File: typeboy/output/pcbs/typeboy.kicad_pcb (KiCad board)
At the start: 2 copper layers, 141.2 x 105.6 mm, 66 parts, among them J2 CartBus

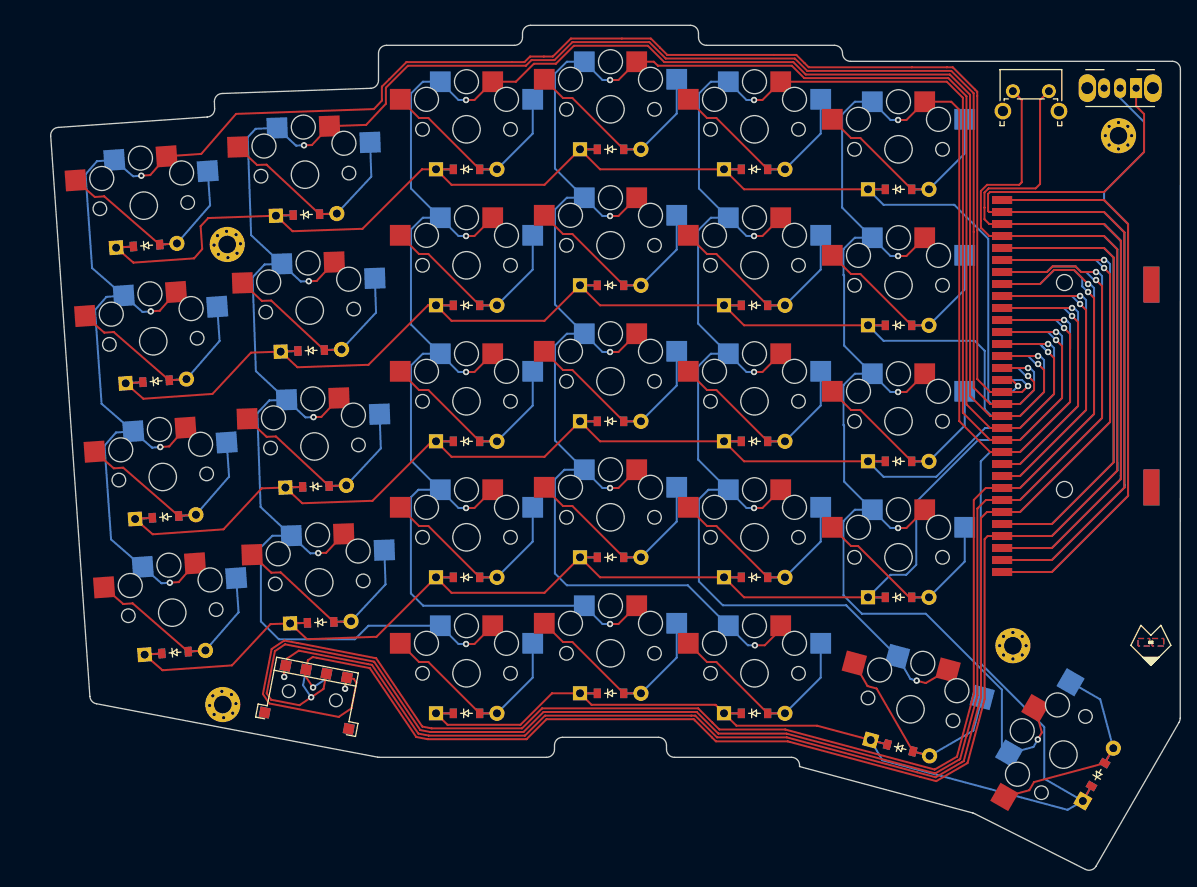
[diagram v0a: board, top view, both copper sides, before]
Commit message: Updated Documentation.
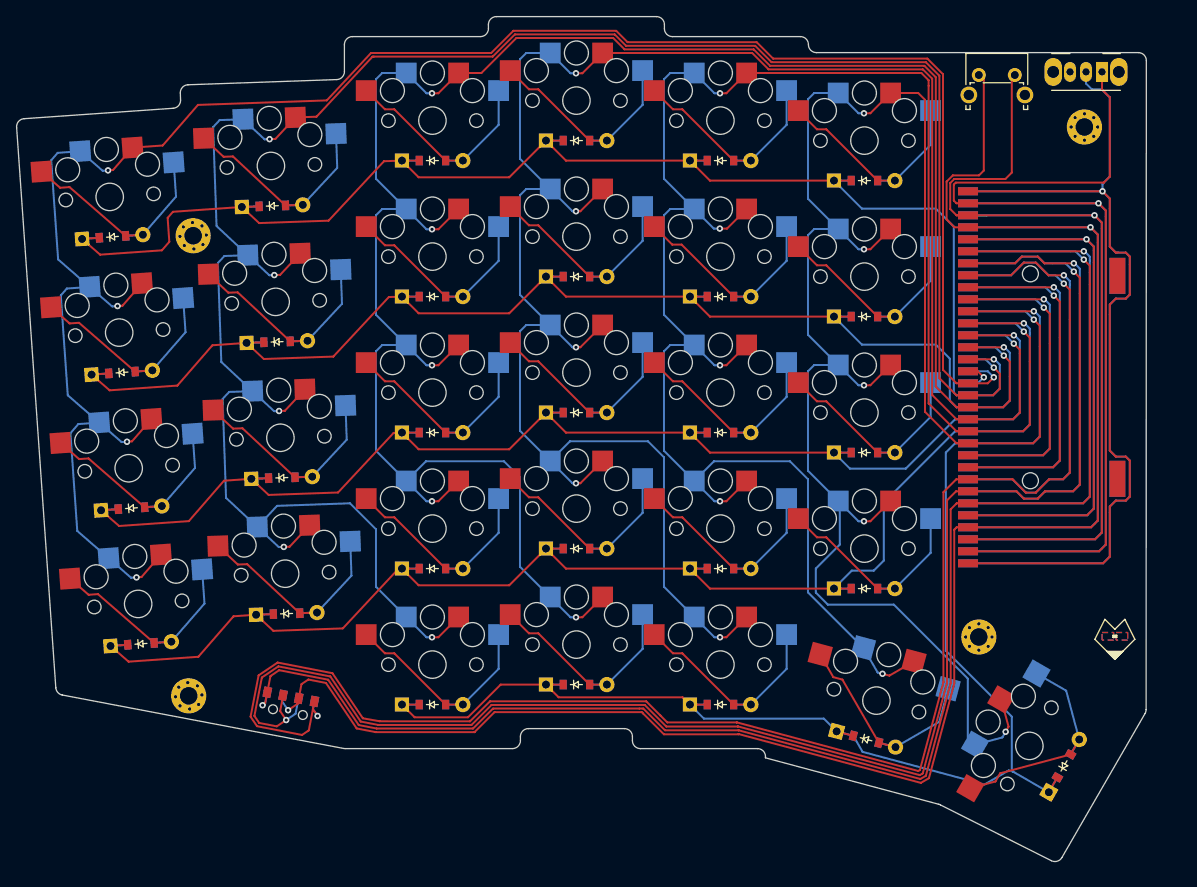
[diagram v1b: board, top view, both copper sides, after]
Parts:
- removed the REF** at (93.2, 192.3)
- added S**: SLLB510100, Custom:SLLB510100, F.Cu at (89.2, 199.5)
- moved REF** 4.71 mm to (176.0, 117.7)
- moved REF** 4.71 mm to (191.4, 117.3)
- moved D12 4.40 mm to (107.7, 145.4)
- moved S27 4.40 mm to (161.7, 125.9)
- moved S7 4.40 mm to (88.1, 146.1)
- moved J2 4.40 mm to (180.4, 155.5)
- moved D16 4.40 mm to (125.7, 159.9)
- moved S3 4.40 mm to (68.5, 149.9)
- moved S25 4.40 mm to (161.7, 159.9)
- moved _1 4.40 mm to (176.0, 188.0)
- moved D19 4.40 mm to (143.7, 196.4)
- moved D28 4.40 mm to (161.9, 200.7)
- moved D10 4.40 mm to (107.7, 179.4)
- moved S15 4.40 mm to (125.7, 171.9)
- moved D9 4.40 mm to (107.7, 196.4)
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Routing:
- net BATOUT: track 158.9 -> 193.2 mm, vias 0 -> 1
- net BATIN: track 168.9 -> 191.1 mm, vias 0 -> 1
- net RST: track 156.8 -> 176.6 mm, vias 0 -> 1
- net VCC: track 114.3 -> 129.8 mm, vias 0 -> 1
- net GND: track 274.9 -> 287.3 mm, vias 1 -> 2
- net MISO: track 247.9 -> 257.6 mm
- net MOSI: track 51.6 -> 61.1 mm
- net NFC1: track 181.3 -> 190.7 mm
- net SCK: track 44.2 -> 52.7 mm
- net col7: track 37.6 -> 43.9 mm
- net IO_CS: track 38.4 -> 44.6 mm
- net col1: track 284.6 -> 279.1 mm
- net col6: track 33.2 -> 38.4 mm
- net row5: track 34.0 -> 39.1 mm
- net NFC0: track 195.5 -> 199.5 mm
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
